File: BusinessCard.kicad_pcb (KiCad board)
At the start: 2 copper layers, 89 x 51 mm, 39 parts, among them J1 USB_B, U1 JW5211, U2 JW5211, U3 JW5211, U5 F1C200s, U6 W25Q80DVSNIG, Y1 24MHz

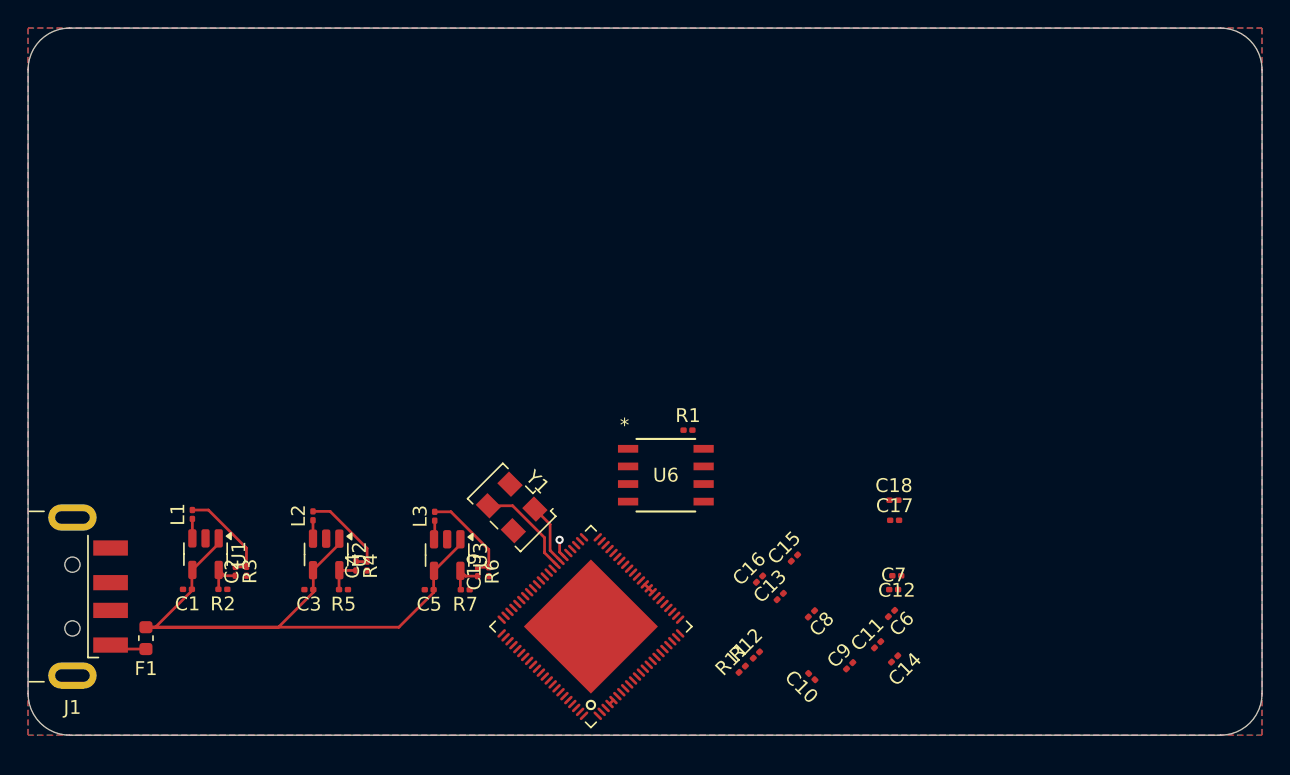
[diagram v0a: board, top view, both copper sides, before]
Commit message: progress
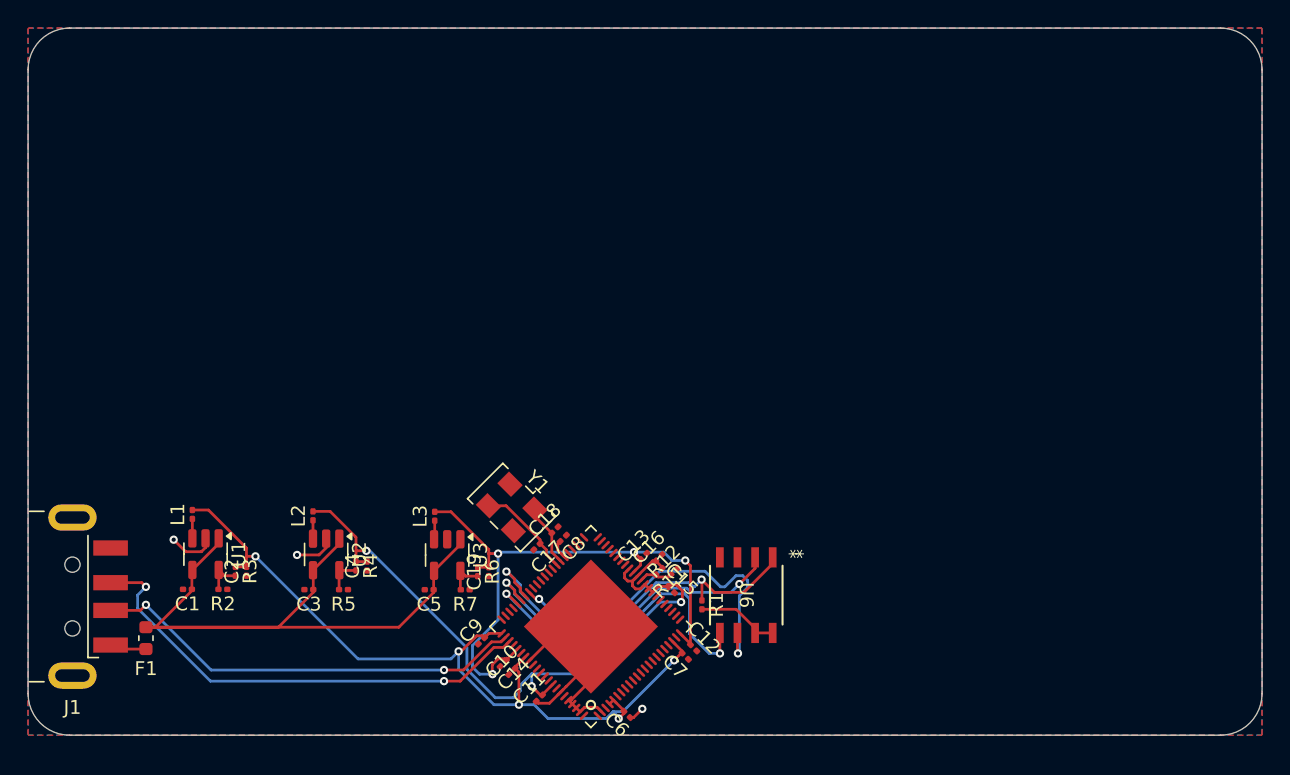
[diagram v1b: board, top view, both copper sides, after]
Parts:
- moved C14 28.2 mm to (220.8, 113.8)
- moved C9 26.6 mm to (219.2, 112.2)
- moved C17 25.9 mm to (223.2, 105.4), turned to -135 degrees
- moved C11 24.7 mm to (223.4, 116.3)
- moved C18 24.5 mm to (224.5, 104.2), turned to 45 degrees
- moved C10 21.6 mm to (221.4, 114.4), turned to 45 degrees
- moved C6 20.4 mm to (229.7, 117.5), turned to 135 degrees
- moved C8 18.7 mm to (225.1, 104.8)
- moved C7 15.8 mm to (233.9, 113.3), turned to 135 degrees
- moved C12 15.6 mm to (234.5, 112.7), turned to -45 degrees
- moved R1 12.6 mm to (235.1, 109.6), turned to -90 degrees
- moved U6 10.4 mm to (238.3, 108.9), turned to -90 degrees
- moved C13 10.3 mm to (230.9, 106.1)
- moved R11 9.26 mm to (232.0, 107.2), turned to -135 degrees
- moved C15 9.16 mm to (232.9, 108.5), turned to -45 degrees
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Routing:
- net +3V3: track 8.97 -> 65.7 mm, vias 1 -> 5
- net +2V5: track 7.56 -> 51.9 mm, vias 0 -> 3
- net +1V1: track 7.10 -> 44.5 mm, vias 0 -> 4
- net USB_DP: track 0.00 -> 34.7 mm, vias 0 -> 2
- net USB_DN: track 0.00 -> 31.6 mm, vias 0 -> 2
- net GND: track 0.00 -> 29.9 mm, vias 0 -> 3
- net SPI_CS: track 0.00 -> 27.5 mm, vias 0 -> 2
- net SPI_CLK: track 0.00 -> 25.2 mm, vias 0 -> 2
- net SPI_MISO: track 0.00 -> 23.4 mm, vias 0 -> 2
- net SPI_MOSI: track 0.00 -> 23.0 mm, vias 0 -> 2
- net Net-(U5B-SVREF): track 0.00 -> 2.48 mm
